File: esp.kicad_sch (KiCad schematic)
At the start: 98 parts, among them J1 Barrel_Jack, J11 Barrel_Jack, J12 Barrel_Jack, J13 Barrel_Jack, J14 Barrel_Jack, J2 8P8C_Shielded, J21 8P8C_Shielded, J27 Barrel_Jack, J3 Barrel_Jack, J38 8P8C_Shielded, J39 Barrel_Jack, J4 Barrel_Jack, J40 Barrel_Jack, J5 Barrel_Jack, J7 Barrel_Jack_MountingPin, K1 RT314A24, K5 RT314A24, P1 Conn_WallPlug_Earth, Q3 MOSFET-NCHANNELSMD, Q4 MOSFET-NCHANNELSMD, Q5 MOSFET-NCHANNELSMD, U1 ESP32-S2-WROVER, U14 L298N, U15 PCF8574ATS, U16 L298N, U17 L298N, U18 NID30S48-24, U19 PCA9685PW, U2 TCA9548ARGER, U20 PCF8574ATS, U3 TCA9548ARGER, U4 BME280, U5 PCF8574ATS, U6 L298N, U7 OKI-78SR-12_1.0-W36H-C, U8 OKI-78SR-5_1.5-W36-C, U9 OKI-78SR-3.3_1.5-W36H-C

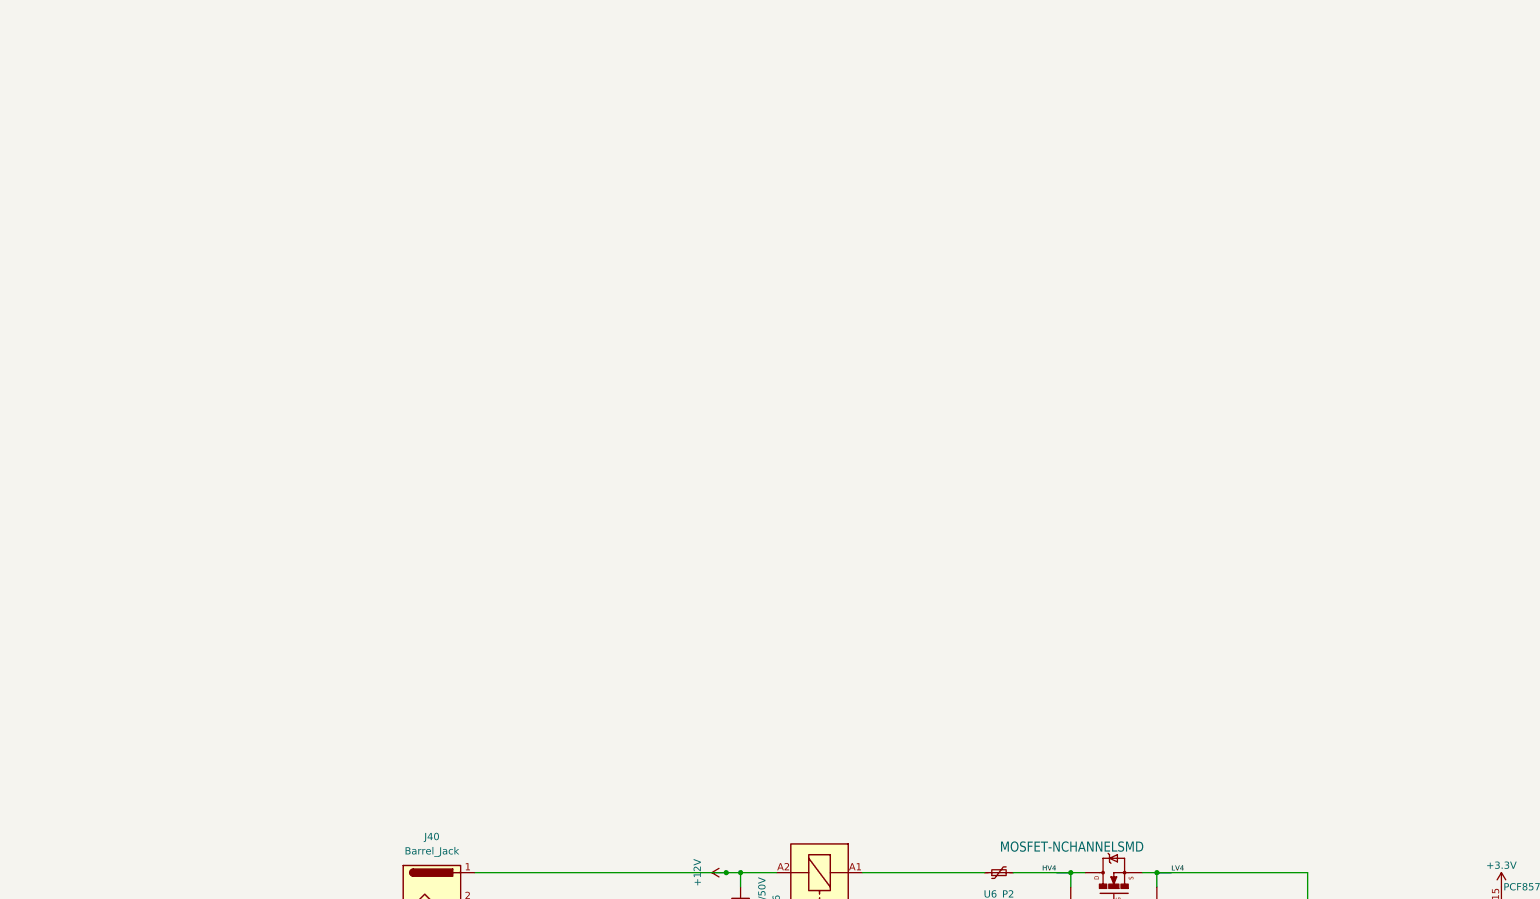
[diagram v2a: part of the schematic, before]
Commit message: relay from SolderedElectronics/2-channel-relay-board-hardware-design
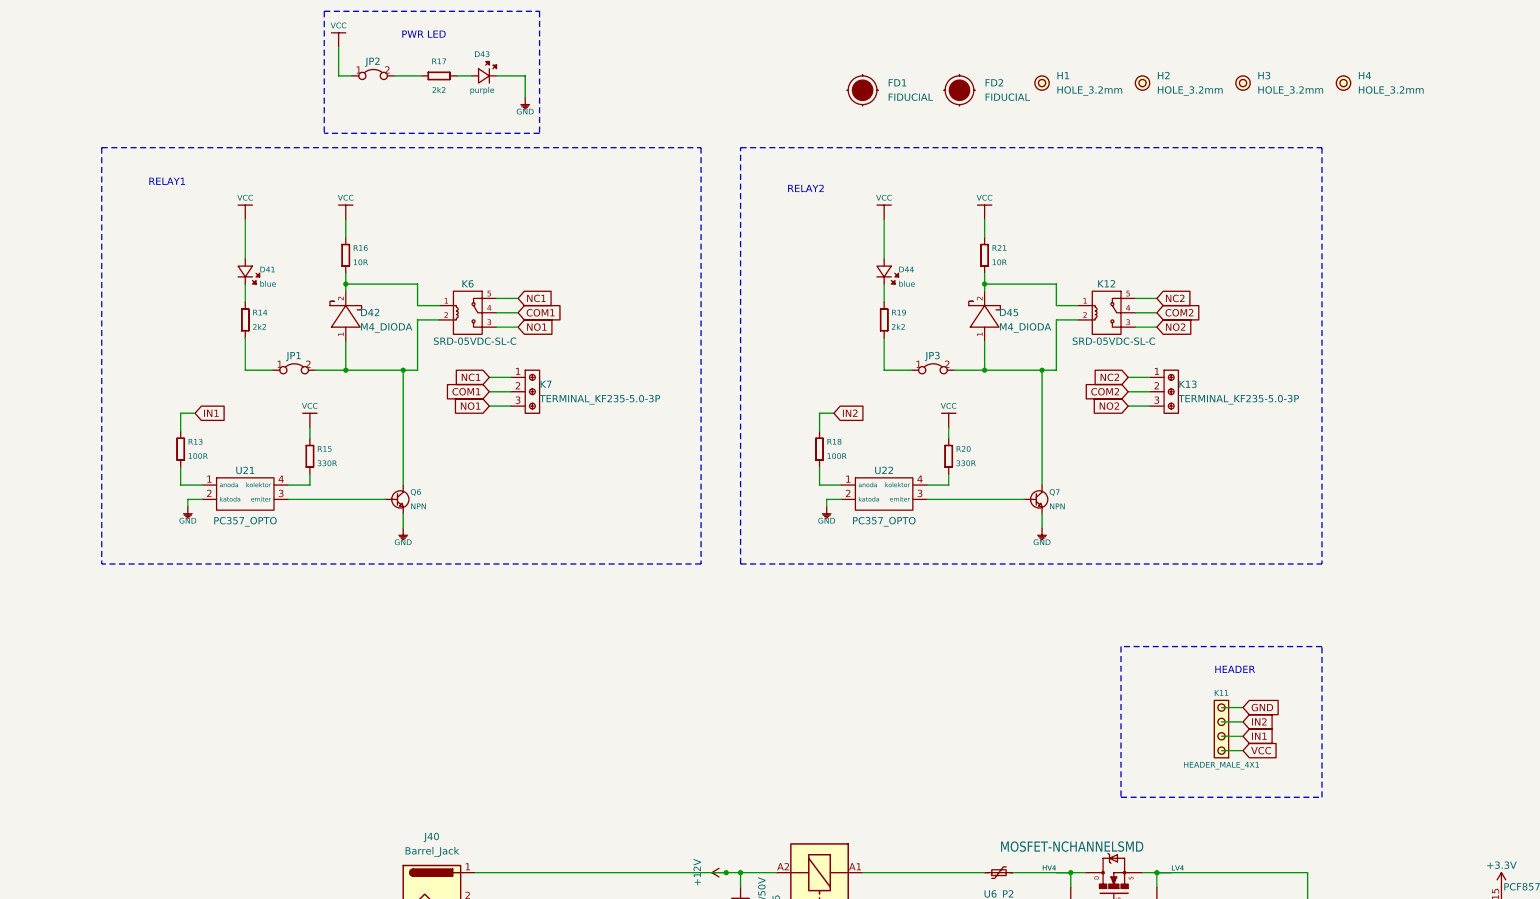
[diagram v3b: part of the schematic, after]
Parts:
- added D41, D44: blue, e-radionica.com footprinti:0402LED, symbol e-radionica.com schematics:0402LED
- added D42, D45: M4_DIODA, e-radionica.com footprinti:M4_DIODA, symbol e-radionica.com schematics:M4_DIODA
- added D43: purple, e-radionica.com footprinti:0402LED, symbol e-radionica.com schematics:0402LED
- added FD1, FD2: FIDUCIAL, e-radionica.com footprinti:FIDUCIAL_23, symbol e-radionica.com schematics:FIDUCIAL
- added H1, H2, H3, H4: HOLE_3.2mm, e-radionica.com footprinti:HOLE_3.2mm, symbol e-radionica.com schematics:HOLE_3.2mm
- added JP1, JP2, JP3: SMD-JUMPER-CONNECTED_TRACE_SLODERMASK, e-radionica.com footprinti:SMD-JUMPER-CONNECTED_TRACE_SLODERMASK, symbol e-radionica.com schematics:SMD-JUMPER-CONNECTED_TRACE_SLODERMASK
- added K11: HEADER_MALE_4X1, e-radionica.com footprinti:HEADER_MALE_4X1, symbol e-radionica.com schematics:HEADER_MALE_4X1
- added K12, K6: SRD-05VDC-SL-C, e-radionica.com footprinti:SRD_RELAY_5V, symbol e-radionica.com schematics:SRD_RELAY_5V
- added K13, K7: TERMINAL_KF235-5.0-3P, e-radionica.com footprinti:TERMINAL_KF235-5.0-3P, symbol e-radionica.com schematics:TERMINAL_KF235-5.0-3P
- added Q6, Q7: NPN, e-radionica.com footprinti:SOT-23-3, symbol e-radionica.com schematics:NPN-SOT-23-3
- added R13, R18: 100R, e-radionica.com footprinti:0603R, symbol e-radionica.com schematics:0603R
- added R14, R17, R19: 2k2, e-radionica.com footprinti:0402R, symbol e-radionica.com schematics:0402R
- added R15, R20: 330R, e-radionica.com footprinti:0603R, symbol e-radionica.com schematics:0603R
- added R16, R21: 10R, e-radionica.com footprinti:0603R, symbol e-radionica.com schematics:0603R
- added U21, U22: PC357_OPTO, e-radionica.com footprinti:PC357_OPTO, symbol e-radionica.com schematics:PC357_OPTO
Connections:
- net GND: now also D43.2 (K), K11.4, Q6.2 (E), Q7.2 (E), U21.2 (katoda), U22.2 (katoda)
- new net: D44.2 (K), R19.2
- new net: R18.1, U22.1 (anoda)
- new net: Q7.1 (B), U22.3 (emiter)
- new net: R20.1, U22.4 (kolektor)
- new net: JP1.1, R14.1
- new net: D41.2 (K), R14.2
- new net: D42.2 (K), K6.1, R16.1
- new net: D42.1 (A), JP1.2, K6.2, Q6.3 (C)
- new net: JP3.1, R19.1
- new net: D43.1 (A), R17.2
- new net: D45.1 (A), JP3.2, K12.2, Q7.3 (C)
- new net: JP2.2, R17.1
- new net: D45.2 (K), K12.1, R21.1
- new net: R13.1, U21.1 (anoda)
- new net: Q6.1 (B), U21.3 (emiter)
- new net: R15.1, U21.4 (kolektor)
- new net COM1: K6.4, K7.2
- new net COM2: K12.4, K13.2
- new net IN1: K11.2, R13.2
- new net IN2: K11.3, R18.2
- new net NC1: K6.5, K7.1
- new net NC2: K12.5, K13.1
- new net NO1: K6.3, K7.3
- new net NO2: K12.3, K13.3
- new net VCC: D41.1 (A), D44.1 (A), JP2.1, K11.1, R15.2, R16.2, R20.2, R21.2
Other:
- note added: "HEADER"
- note added: "PWR LED"
- note added: "RELAY1"
- note added: "RELAY2"
